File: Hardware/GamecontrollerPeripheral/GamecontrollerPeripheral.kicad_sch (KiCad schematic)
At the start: 13 parts, among them J2 UPDI, SW1 Joystick, SW6 DPad, U1 ATtiny1604-SS

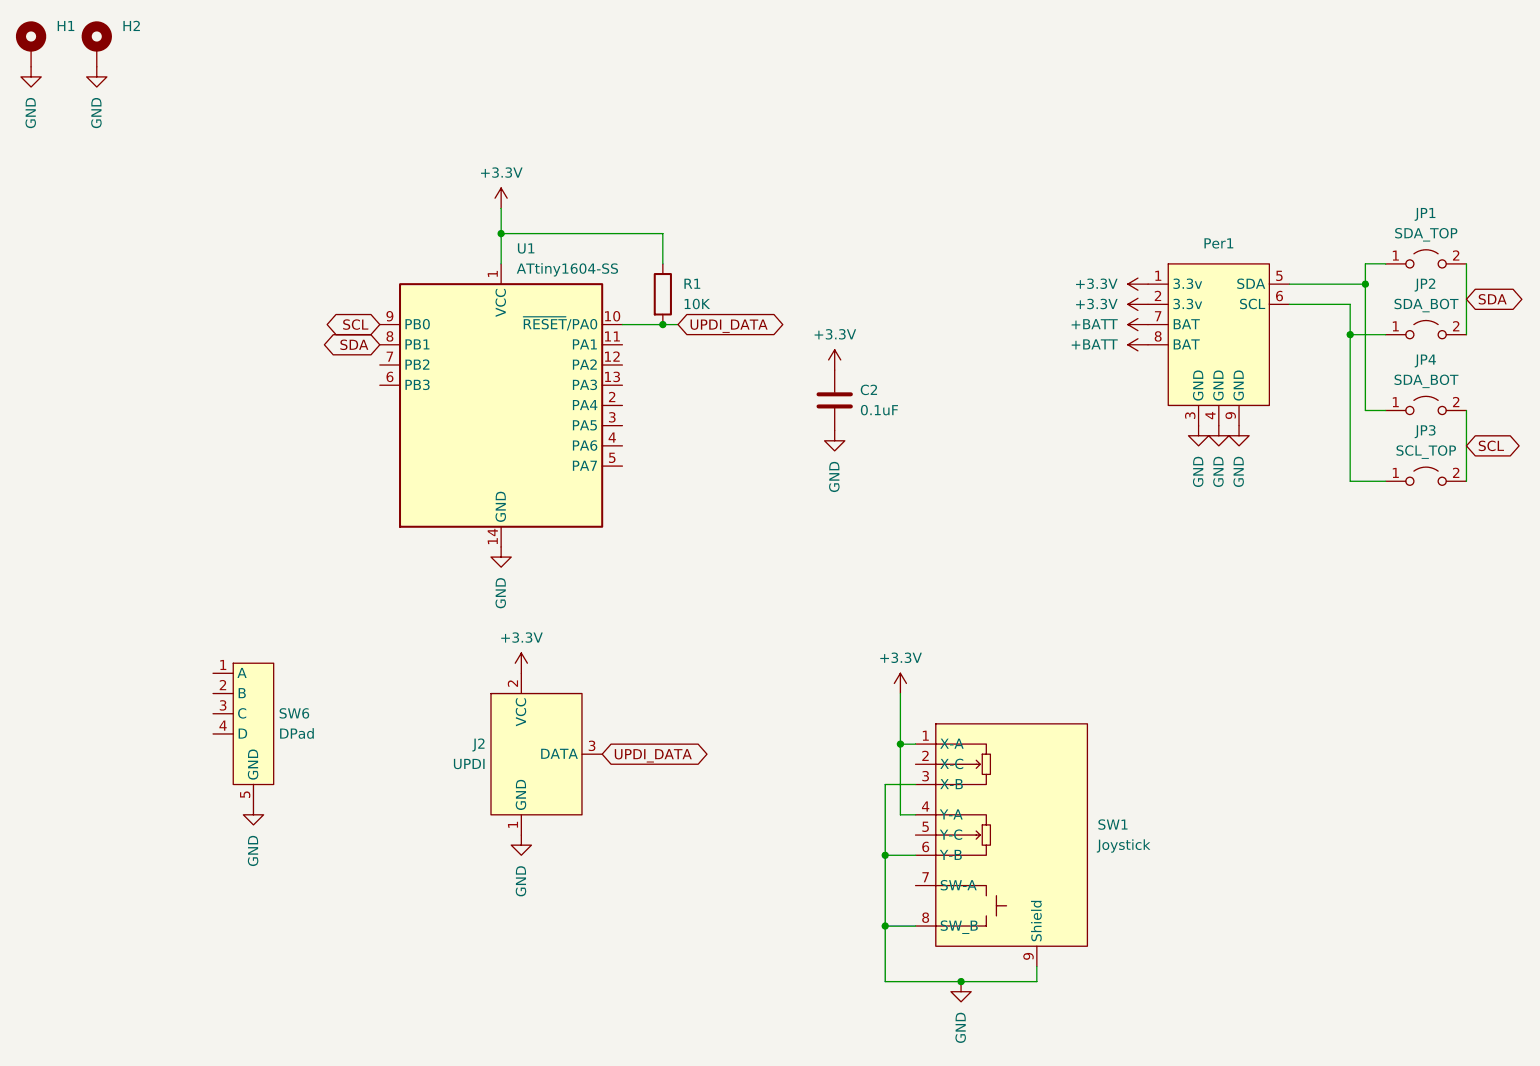
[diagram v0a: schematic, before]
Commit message: GamecontrollerPeripheral progres
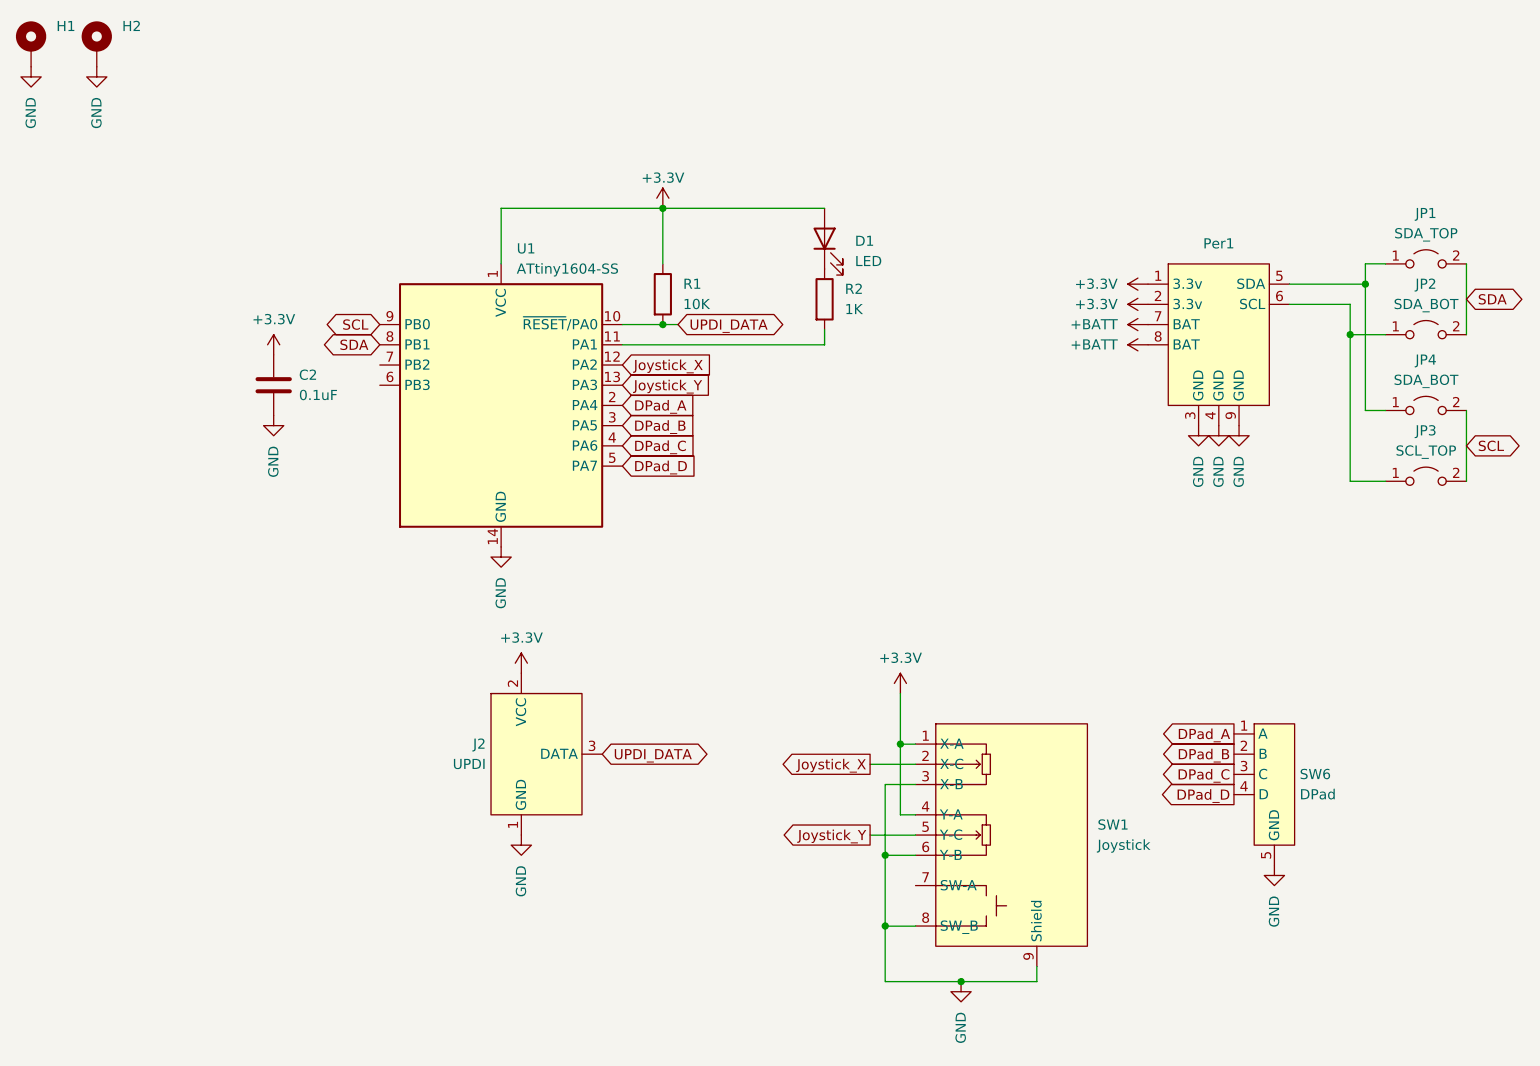
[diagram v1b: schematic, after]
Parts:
- added D1: LED, LED_SMD:LED_0805_2012Metric_Pad1.15x1.40mm_HandSolder, symbol Device:LED
- added R2: 1K, Resistor_SMD:R_0805_2012Metric_Pad1.20x1.40mm_HandSolder, symbol Device:R
- C2: footprint (none) -> Capacitor_SMD:C_0805_2012Metric_Pad1.18x1.45mm_HandSolder
- R1: footprint (none) -> Resistor_SMD:R_0805_2012Metric_Pad1.20x1.40mm_HandSolder
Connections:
- net +3.3V: now also D1.2 (A)
- net DPad_A: now reaches SW6.1 (A)
- net DPad_A: now also U1.2 (PA4)
- net DPad_B: now reaches SW6.2 (B)
- net DPad_B: now also U1.3 (PA5)
- net DPad_C: now reaches SW6.3 (C)
- net DPad_C: now also U1.4 (PA6)
- net DPad_D: now reaches SW6.4 (D)
- net DPad_D: now also U1.5 (PA7)
- net at U1.11 (PA1): now also R2.2
- net Joystick_X: now reaches U1.12 (PA2)
- net Joystick_X: now also SW1.2 (X-C)
- net Joystick_Y: now reaches U1.13 (PA3)
- net Joystick_Y: now also SW1.5 (Y-C)
- new net: D1.1 (K), R2.1
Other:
- moved on the sheet: C2, SW6
